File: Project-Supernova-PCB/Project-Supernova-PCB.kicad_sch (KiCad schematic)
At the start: 38 parts, among them J1 Conn_01x04, J10 Conn_01x02, J11 Screw_Terminal_01x02, J12 Screw_Terminal_01x02, J2 Conn_01x04, J3 Conn_01x02, J4 Conn_Coaxial, J6 100k_Thermistor, J6 Screw_Terminal_01x02, J7 100k_Thermistor, J7 Screw_Terminal_01x02, J9 Conn_01x02, Q1 AO3420, SW1 SW_SPDT, SW2 SW_SPDT, U1 GY-NEO6MV2-Module, U2 BMP280-Module, U3 LoRa-E5, U4 LM335D, U5 ESP32-Module-30Pin, U6 S09

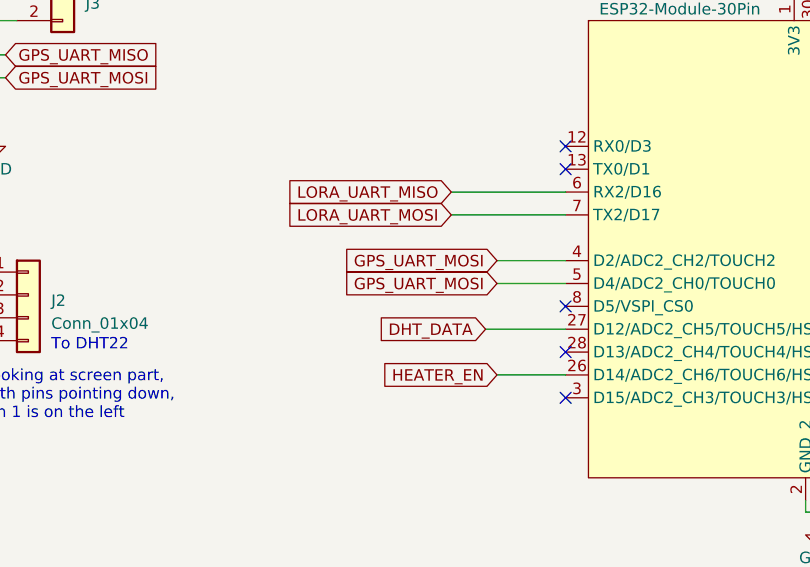
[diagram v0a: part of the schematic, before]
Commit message: Routed PCB
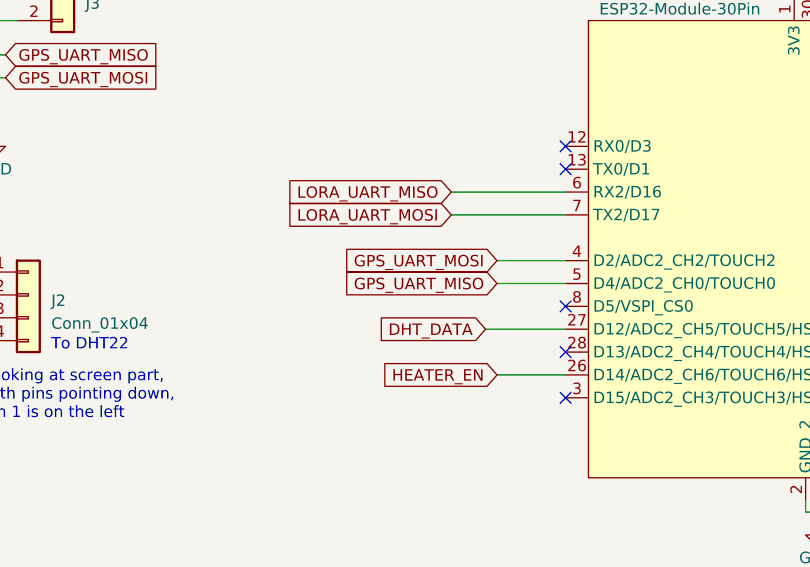
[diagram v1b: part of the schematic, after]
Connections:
- net GPS_UART_MISO: now also U5.5 (D4/ADC2_CH0/TOUCH0)
- net GPS_UART_MOSI: no longer U5.5 (D4/ADC2_CH0/TOUCH0)
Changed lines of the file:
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@@
-    )
-  )
-  (global_label "GPS_UART_MOSI" (shape input) (at 113.03 95.25 180) (fields_autoplaced)
-    (effects (font (size 1.27 1.27)) (justify right))
-    (property "Intersheetrefs" "${INTERSHEET_REFS}" (at 95.1866 95.25 0)
-      (effects (font (size 1.27 1.27)) (justify right) hide)
     )
   )
@@
       (effects (font (size 1.27 1.27)) (justify right) hide)
     )
+  )
+  (global_label "GPS_UART_MISO" (shape input) (at 113.03 95.25 180) (fields_autoplaced)
+    (effects (font (size 1.27 1.27)) (justify right))
+    (property "Intersheetrefs" "${INTERSHEET_REFS}" (at 95.1866 95.25 0)
+      (effects (font (size 1.27 1.27)) (justify right) hide)
+    )
